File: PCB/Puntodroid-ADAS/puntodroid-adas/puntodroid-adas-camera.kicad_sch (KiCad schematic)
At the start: 26 parts, among them J4 RCA_SOCKET, J5 VIDEO_OUTPUT, U3 AT7456, U4 PI5V330, U5 THS7373, Y2 27MHz

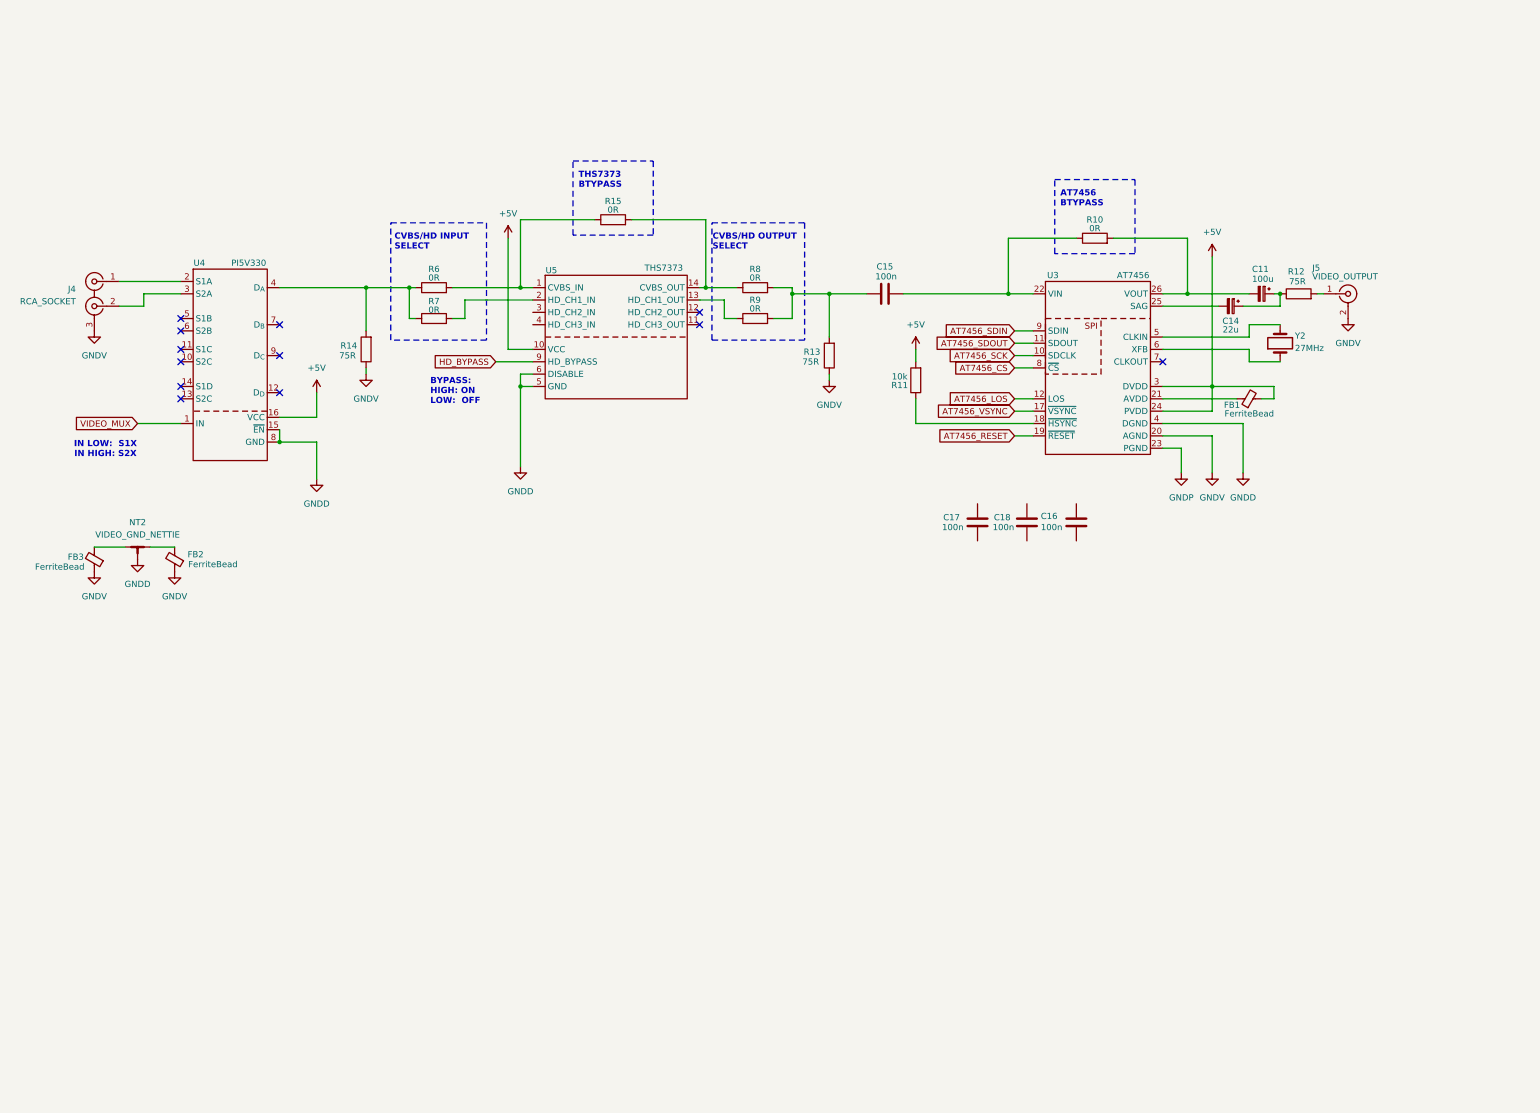
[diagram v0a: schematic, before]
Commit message: update puntodroid schematic
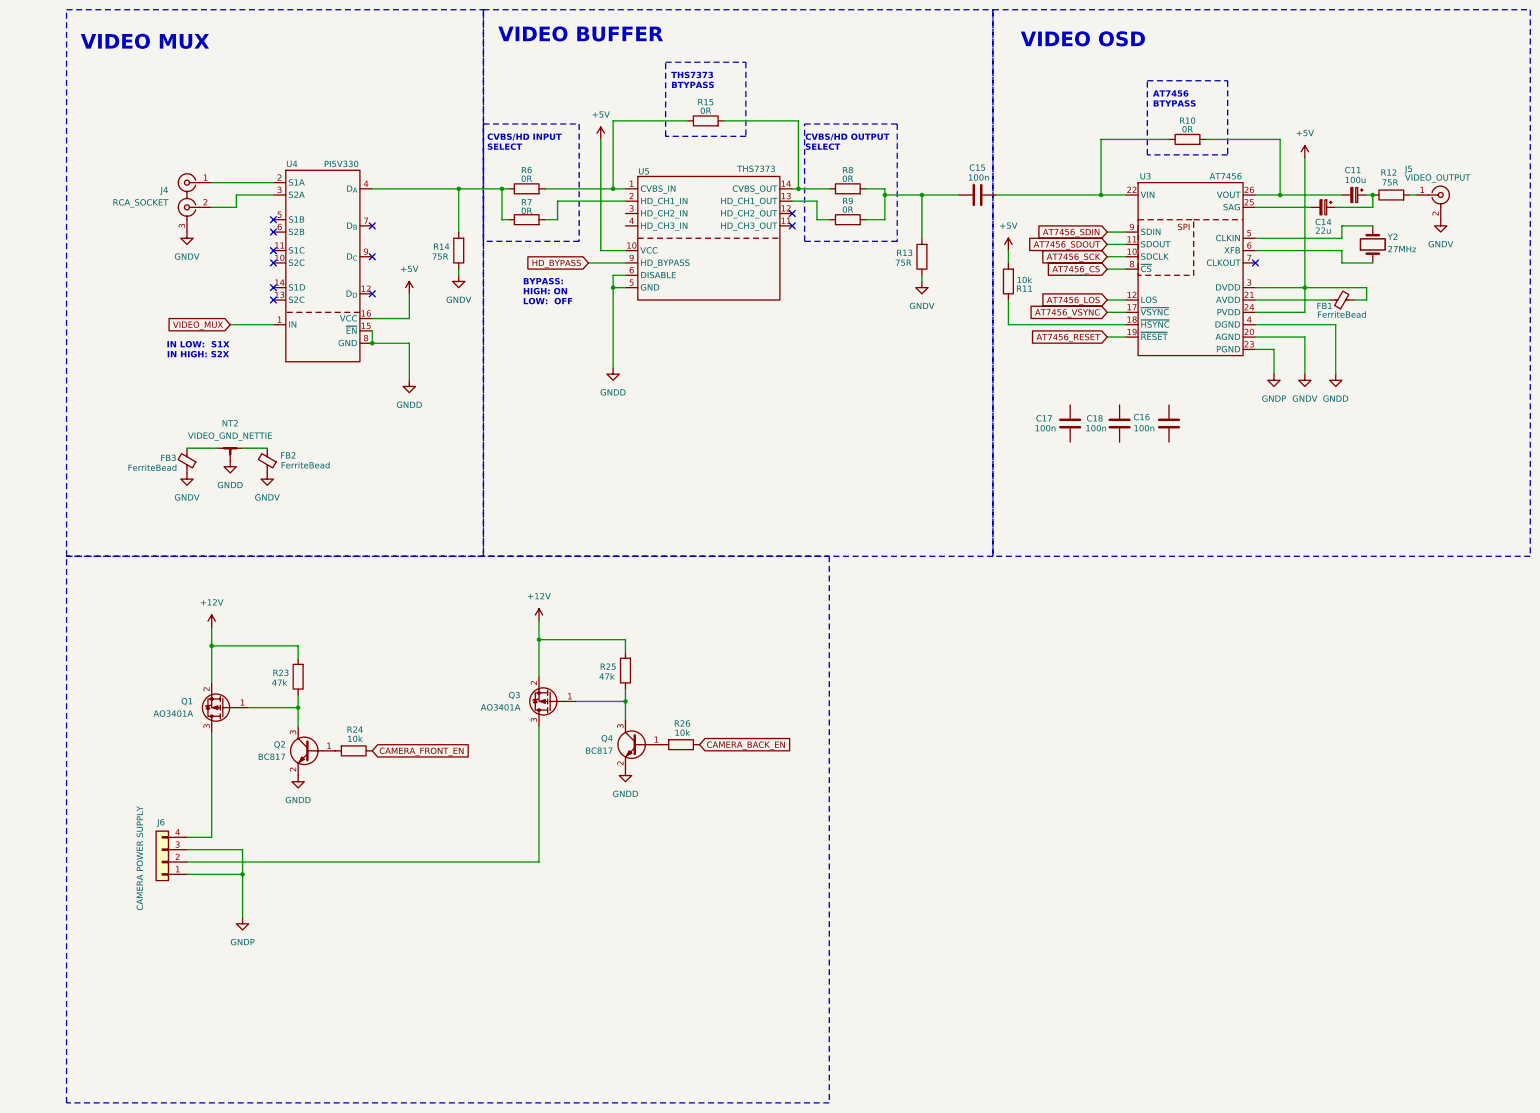
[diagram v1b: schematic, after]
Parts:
- added J6: CAMERA POWER SUPPLY, symbol Connector_Generic:Conn_01x04
- added Q1, Q3: AO3401A, Package_TO_SOT_SMD:SOT-23, symbol Transistor_FET:AO3401A
- added Q2, Q4: BC817, Package_TO_SOT_SMD:SOT-23, symbol Transistor_BJT:BC817
- added R23, R25: 47k, symbol Device:R
- added R24, R26: 10k, symbol Device:R
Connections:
- net GNDD: now also Q2.2 (E), Q4.2 (E)
- net GNDP: now also J6.1 (Pin_1), J6.3 (Pin_3)
- new net: Q2.1 (B), R24.2
- new net: Q1.1 (G), Q2.3 (C), R23.1
- new net: J6.4 (Pin_4), Q1.3 (D)
- new net: J6.2 (Pin_2), Q3.3 (D)
- new net: Q4.1 (B), R26.2
- new net: Q3.1 (G), Q4.3 (C), R25.1
- new net +12V: Q1.2 (S), Q3.2 (S), R23.2, R25.2
- new net CAMERA_BACK_EN: R26.1
- new net CAMERA_FRONT_EN: R24.1
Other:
- note added: "VIDEO BUFFER"
- note added: "VIDEO MUX"
- note added: "VIDEO OSD"
- moved on the sheet: C11, C14, C15, C16, C17, C18, FB1, FB2, FB3, J4, J5, NT2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
